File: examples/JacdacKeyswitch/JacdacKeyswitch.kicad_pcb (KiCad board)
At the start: 2 copper layers, 35 x 25 mm, 39 parts

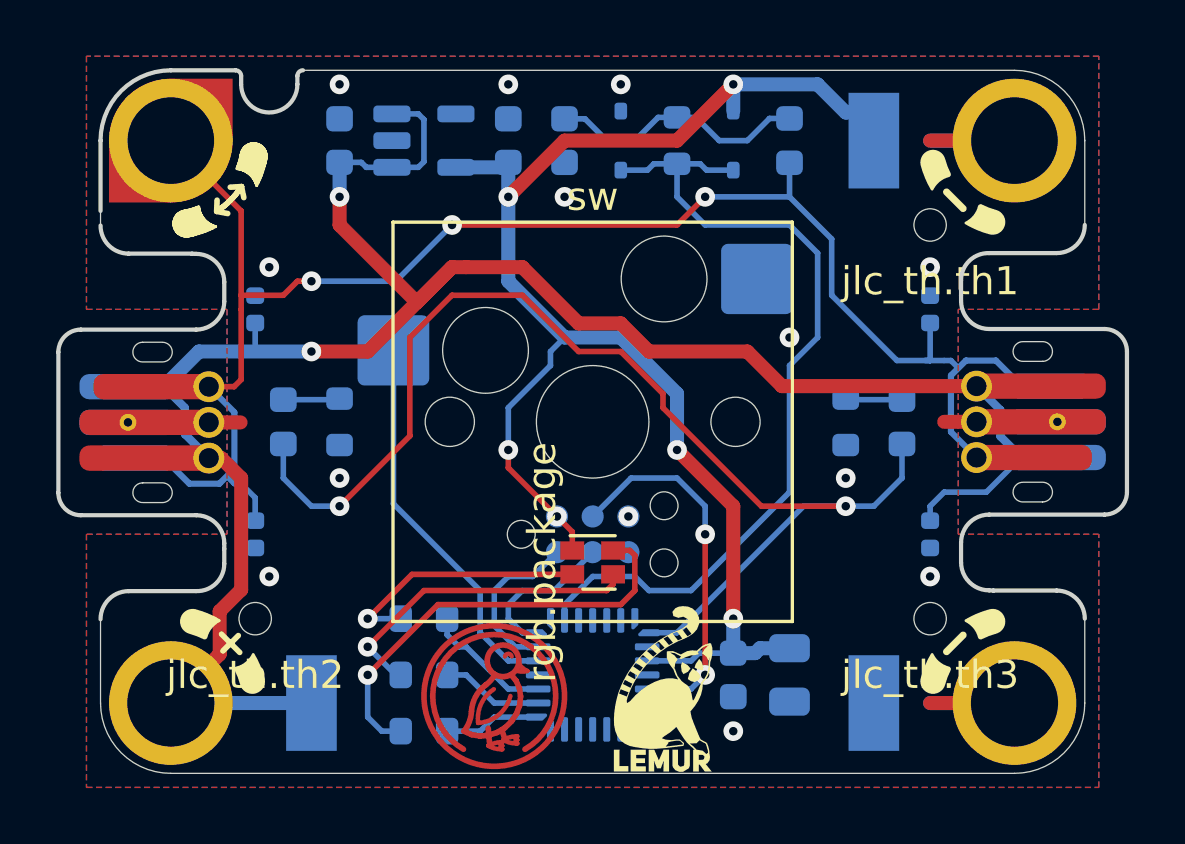
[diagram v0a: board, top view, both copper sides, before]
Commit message: layout rc1
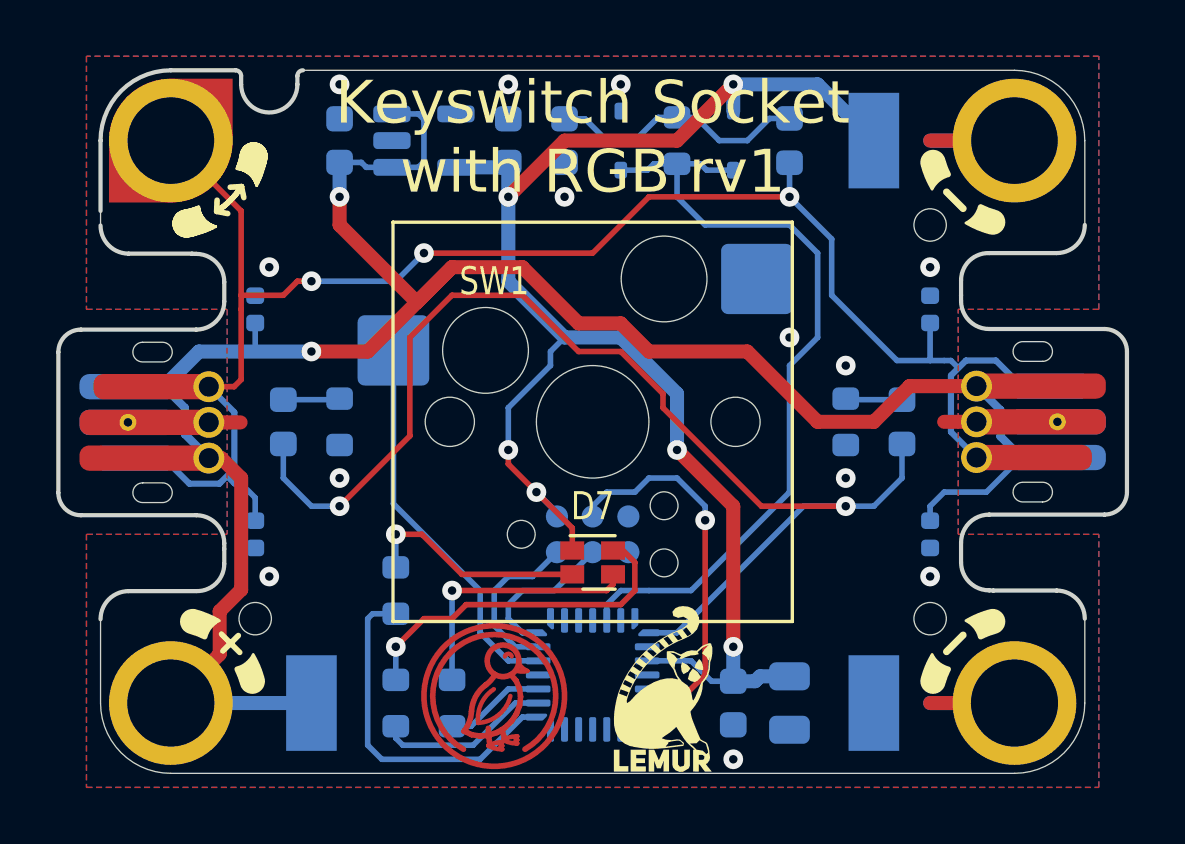
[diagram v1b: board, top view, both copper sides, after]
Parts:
- moved R3 1.41 mm to (143.0, 110.0), turned to -90 degrees
- moved R4 1.41 mm to (145.0, 110.0), turned to -90 degrees
- moved R5 1.41 mm to (143.0, 106.0), turned to -90 degrees
- moved C3 1.00 mm to (157.0, 110.0)
- moved C4 1.00 mm to (155.0, 110.0)
- renumbered reg_3v3.in_cap to C1, reg_3v3.out_cap to C2, mcu.pwr_cap0 to C3, mcu.pwr_cap1 to C4, jd_if.rc.c to C5, edge.status_led.package to D1, edge.tvs_jd_pwr to D2, edge.tvs_jd_data to D3, edge2.status_led.package to D4, edge2.tvs_jd_pwr to D5, edge2.tvs_jd_data to D6, rgb.package to D7, jd_if.clamp_hi to D8, jd_if.clamp_lo to D9, edge.conn to EC1, edge2.conn to EC2, jd_if.ferrite to FB1, jlc_th.th1 to H1, jlc_th.th2 to H2, jlc_th.th3 to H3, mcu.swd to J1, jd_mh1 to MH1, jd_mh2 to MH2, jd_mh3 to MH3, jd_mh4 to MH4, edge.status_led.res to R1, edge2.status_led.res to R2, rgb.red_res to R3, rgb.green_res to R4, rgb.blue_res to R5, jd_if.rc.r to R6, sw to SW1, tp_jd_pwr to TP1, tp_gnd to TP2, tp_3v3 to TP3, reg_3v3.ic to U1, mcu.ic to U2
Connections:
- U2 pad 15: rgb.signals.red -> rgb.signals.blue
- U2 pad 16: rgb.signals.green -> rgb.signals.red
- U2 pad 17: rgb.signals.blue -> rgb.signals.green
- U2 pad 23: jd_if.signal -> (no net)
- U2 pad 26: (no net) -> jd_if.signal
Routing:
- net rgb.signals.blue: track 4.61 -> 12.4 mm
- net rgb.red_res.a: track 15.7 -> 12.5 mm
- net rgb.signals.red: track 3.38 -> 6.21 mm
- net v3v3: track 54.5 -> 56.8 mm
- net rgb.green_res.a: track 11.6 -> 9.34 mm
- net jd_if.signal: track 30.7 -> 28.8 mm
- net rgb.blue_res.a: track 9.10 -> 8.04 mm
- net jd_pwr: track 71.7 -> 72.7 mm
- net mcu.reset_node: track 13.2 -> 13.9 mm
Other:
- board text added: "Keyswitch Socket with RGB rv1"
